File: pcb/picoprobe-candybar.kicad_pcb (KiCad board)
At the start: 2 copper layers, 27.9 x 102.4 mm, 35 parts, among them J0 SWD-UART_PicoprobeCandybar, J1 PinHeader_2x04, J2 PinSocket_1x03, J3 PinSocket_1x03, J4 PinSocket_1x03, J5 PinSocket_1x03, J6 PinSocket_1x03, J7 PinSocket_1x03, Q1 T2N7002AK, Q2 DMP31D1U, SW1 SW-R1-1A-E-1-0, SW2 SLW-156646-5A-N-D, SW3 SLW-1277545-2A-RA-S-D, U1 TLV77318PDBVR, U2 TLV77325PDBVR, U3 SN74LV6T17, U4 SN74LV6T17

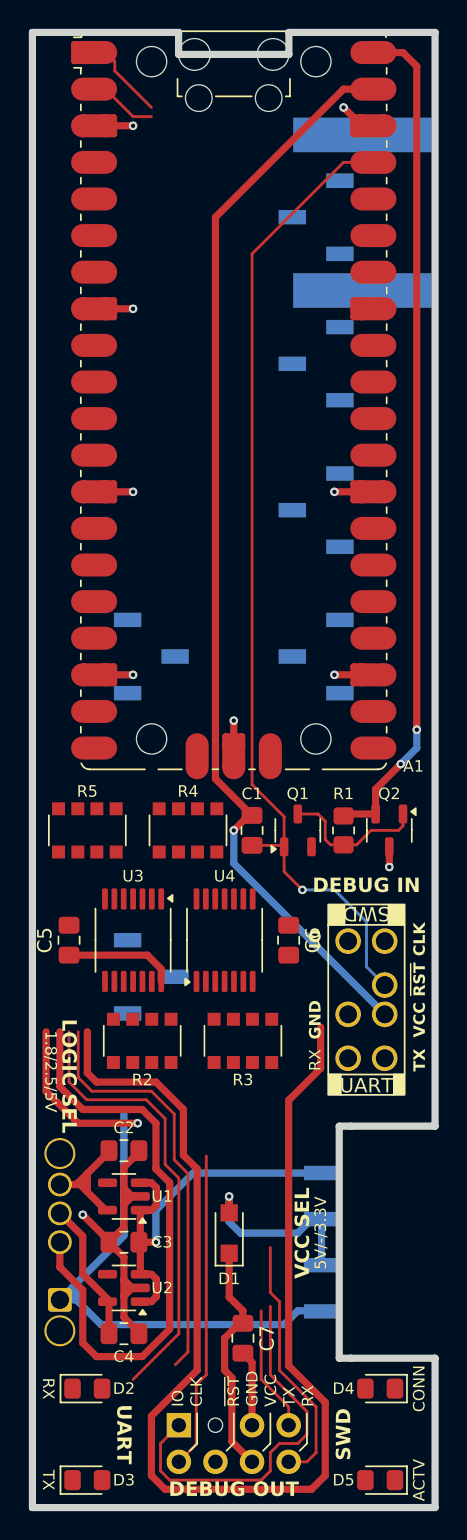
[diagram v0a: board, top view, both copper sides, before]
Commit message: Major in-progress layout redesign
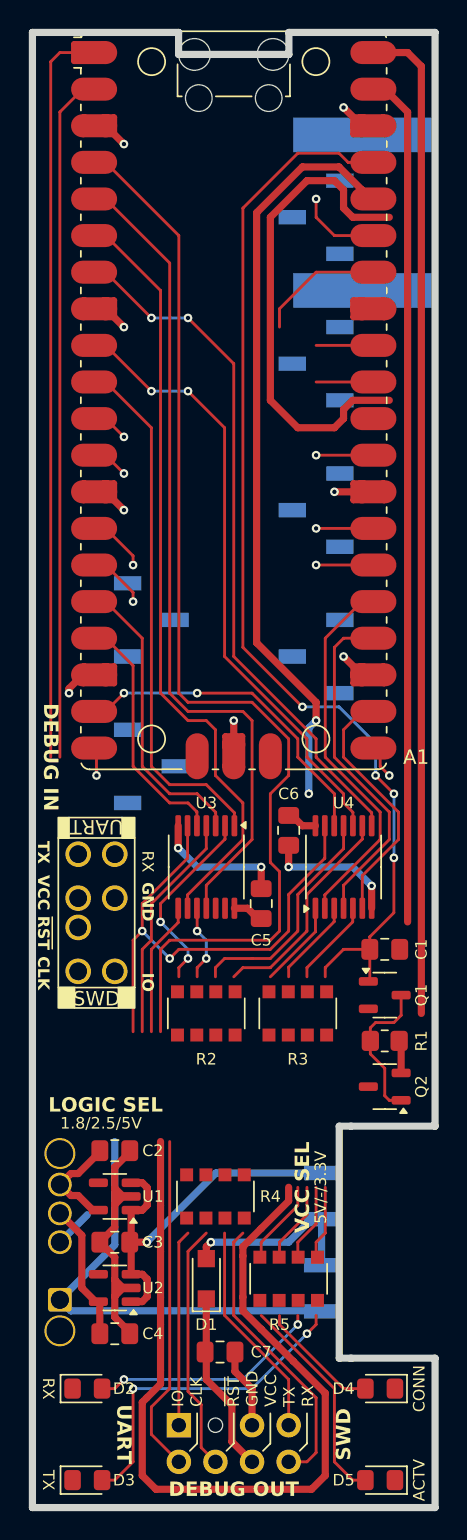
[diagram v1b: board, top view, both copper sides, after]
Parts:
- A1: footprint Module_RaspberryPi_Pico:RaspberryPi_Pico_Original_SMD_MountingHoles_HandSolder -> Module_RaspberryPi_Pico:RaspberryPi_Pico_Original_SMD_HandSolder
- moved R5 34.1 mm to (105.4, 146.7)
- moved R4 25.5 mm to (100.3, 141.0), turned to -90 degrees
- moved Q2 17.8 mm to (112.1, 133.3), turned to 180 degrees
- moved J0 16.3 mm to (93.3, 125.1), turned to 180 degrees
- moved R1 14.9 mm to (112.1, 130.2), turned to 0 degrees
- moved J2 14.6 mm to (95.9, 111.1)
- moved C5 13.6 mm to (103.5, 120.7)
- moved Q1 12.9 mm to (112.1, 127.0), turned to 0 degrees
- moved C1 12.4 mm to (112.1, 123.8), turned to 180 degrees
- moved U4 9.69 mm to (109.2, 118.1)
- moved C6 7.62 mm to (105.4, 115.6)
- moved U3 7.18 mm to (99.7, 118.1)
- moved R2 4.84 mm to (99.7, 128.3)
- moved R3 4.26 mm to (106.0, 128.3)
- moved D1 3.55 mm to (99.7, 146.7)
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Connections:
- A1 pad 4: /CB_~{RST} -> /~{RST}
- J2 pad 2: /CB_CTS -> /CB_RTS
- J2 pad 3: /CB_RTS -> /CB_CTS
- J3 pad 1: /INT_RISE -> unconnected-(J3-Pin_1-Pad1)
- J3 pad 3: unconnected-(J3-Pin_3-Pad3) -> /INT_RISE
- R2 pad 1: Net-(R2A-R1.1) -> /CB_RS1
- R2 pad 2: Net-(R2B-R2.1) -> /CB_CTS
- R2 pad 3: Net-(R2C-R3.1) -> /CB_RX
- R2 pad 4: Net-(R2D-R4.1) -> /3V3_EN
- R2 pad 5: /CB_RTS -> Net-(R2D-R4.2)
- R2 pad 6: /CB_TX -> Net-(R2C-R3.2)
- R2 pad 7: /CB_DTR -> Net-(R2B-R2.2)
- R2 pad 8: /3V3_EN -> Net-(R2A-R1.2)
- R3 pad 1: Net-(R3A-R1.1) -> /CB_RTS
- R3 pad 2: Net-(R3B-R2.1) -> /CB_CLK
- R3 pad 3: Net-(R3C-R3.1) -> /CB_DTR
- R3 pad 4: Net-(R3D-R4.1) -> /CB_TX
- R3 pad 5: /CB_CTS -> Net-(R3D-R4.2)
- R3 pad 6: /CB_RX -> Net-(R3C-R3.2)
- R3 pad 7: /CB_IO -> Net-(R3B-R2.2)
- R3 pad 8: /CB_CLK -> Net-(R3A-R1.2)
- R4 pad 1: Net-(R4A-R1.1) -> /~{RST}
- R4 pad 4: Net-(R4D-R4.1) -> /IO_SHIFTED
- R4 pad 5: /CB_RS3 -> /CB_IO
- R4 pad 7: /CB_RS1 -> /CB_RS3
- R4 pad 8: /CB_IO -> /CB_~{RST}
- R5 pad 1: /LED_TX -> /LED_RX
- R5 pad 2: /LED_RX -> /LED_TX
- R5 pad 7: Net-(D3-A) -> Net-(D2-A)
- R5 pad 8: Net-(D2-A) -> Net-(D3-A)
- SW1 pad 2: Net-(R2A-R1.1) -> Net-(R2D-R4.2)
- U3 pad 1: /DTR -> /RTS
- U3 pad 10: Net-(R3A-R1.1) -> Net-(R3C-R3.2)
- U3 pad 11: /CLK -> /DTR
- U3 pad 12: Net-(R3B-R2.1) -> unconnected-(U3-6Y-Pad12)
- U3 pad 13: /IO_OUT -> unconnected-(U3-6A-Pad13)
- U3 pad 2: Net-(R2B-R2.1) -> Net-(R3A-R1.2)
- U3 pad 3: /TX -> /CLK
- U3 pad 4: Net-(R2C-R3.1) -> Net-(R3B-R2.2)
- U3 pad 5: /RTS -> /IO_OUT
- U3 pad 6: Net-(R2D-R4.1) -> /IO_SHIFTED
- U3 pad 8: unconnected-(U3-4Y-Pad8) -> Net-(R3D-R4.2)
- U3 pad 9: unconnected-(U3-4A-Pad9) -> /TX
- U4 pad 1: Net-(R3C-R3.1) -> Net-(R4B-R2.1)
- U4 pad 10: /RS2 -> /CTS
- U4 pad 11: Net-(R4C-R3.1) -> Net-(R2B-R2.2)
- U4 pad 12: /RS3 -> /IO_IN
- U4 pad 13: Net-(R4D-R4.1) -> /IO_SHIFTED
- U4 pad 2: /RX -> /RS3
- U4 pad 3: Net-(R3D-R4.1) -> Net-(R4C-R3.1)
- U4 pad 4: /CTS -> /RS2
- U4 pad 5: Net-(R4A-R1.1) -> Net-(R2A-R1.2)
- U4 pad 6: /IO_IN -> /RS1
- U4 pad 8: /RS1 -> /RX
- U4 pad 9: Net-(R4B-R2.1) -> Net-(R2C-R3.2)
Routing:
- net /~{RST}: track 0.00 -> 76.5 mm
- net /DTR: track 0.00 -> 57.0 mm
- net 3V3: track 28.0 -> 82.9 mm, vias 1 -> 3
- net /TX: track 0.00 -> 53.0 mm
- net /RX: track 0.02 -> 47.5 mm, vias 0 -> 2
- net Net-(A1-GPIO0): track 5.13 -> 52.3 mm
- net Net-(A1-GPIO1): track 3.96 -> 48.6 mm
- net VLOGIC: track 48.7 -> 4.85 mm
- net /CTS: track 0.00 -> 41.9 mm, vias 0 -> 2
- net /RTS: track 0.00 -> 36.0 mm
- net /IO_SHIFTED: track 0.00 -> 35.9 mm, vias 0 -> 2
- net AGND: track 0.00 -> 34.0 mm
- net (no net): track 29.0 -> 0.00 mm
- net /RS3: track 0.00 -> 25.5 mm
- net /RS2: track 0.00 -> 23.2 mm
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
